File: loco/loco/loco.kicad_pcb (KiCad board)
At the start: 2 copper layers, 26 x 11.4 mm, 4 parts, among them U1 STM32F030F4Px, U2 A4953_LJ, U3 TLV760

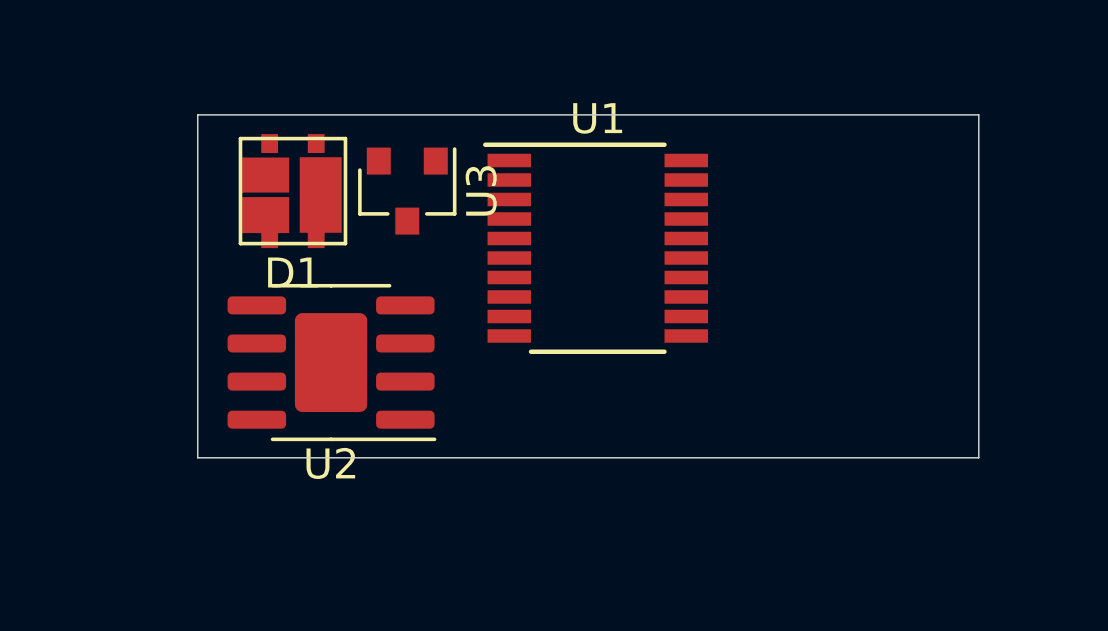
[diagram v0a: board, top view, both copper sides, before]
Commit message: Update
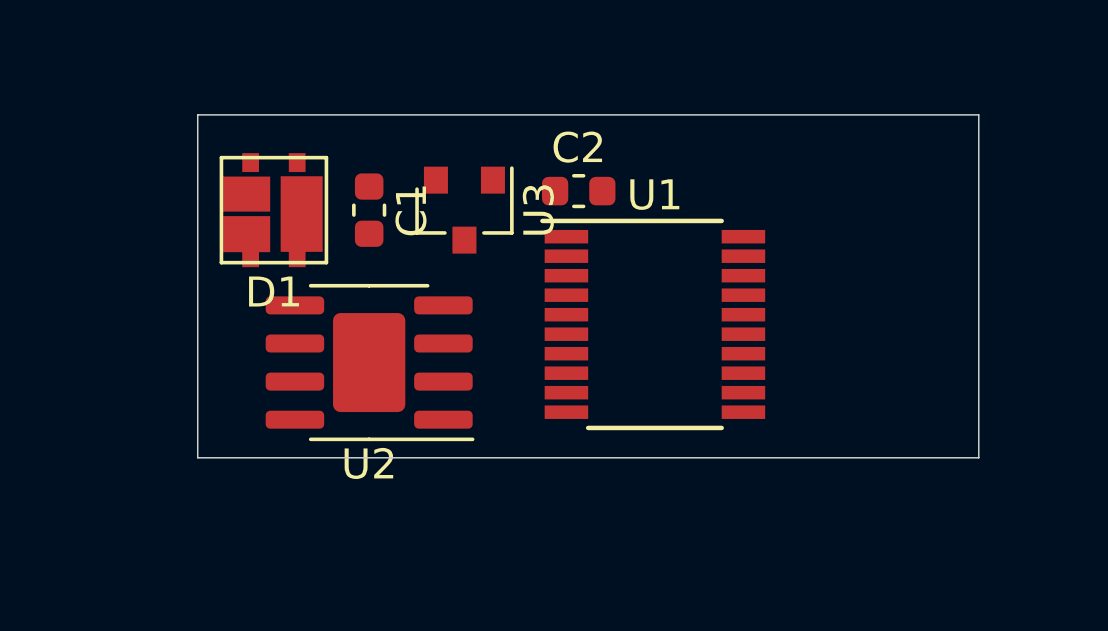
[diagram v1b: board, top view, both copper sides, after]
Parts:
- added C1: C, Capacitor_SMD:C_0603_1608Metric, F.Cu at (121.9, 82.5)
- added C2: C, Capacitor_SMD:C_0603_1608Metric, F.Cu at (128.9, 81.9)
- moved U1 3.18 mm to (131.4, 86.4)
- moved U3 2.01 mm to (125.1, 82.5)
- moved U2 1.27 mm to (121.9, 87.6)
- moved D1 0.90 mm to (118.7, 82.5)
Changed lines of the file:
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@@
     (tracks 0)
     (zones 0)
-    (modules 4)
+    (modules 6)
     (nets 29)
   )
@@
     (add_net RAIL2)
   )
+  (module Capacitor_SMD:C_0603_1608Metric (layer F.Cu)
+    (at 128.905 81.915)
+    (descr "Capacitor SMD 0603 (1608 Metric), square (rectangular) end terminal, IPC_7351 nominal, (Body size source: http://www.tortai-tech.com/upload/download/2011102023233369053.pdf), generated with kicad-footprint-generator")
+    (tags capacitor)
+    (attr smd)
+    (fp_text reference C2 (at 0 -1.43) (layer F.SilkS)
+      (effects (font (size 1 1) (thickness 0.15)))
+    )
+    (fp_text value C (at 0 1.43) (layer F.Fab)
+      (effects (font (size 1 1) (thickness 0.15)))
+    )
+    (fp_text user %R (at 0 0) (layer F.Fab)
+      (effects (font (size 0.4 0.4) (thickness 0.06)))
+    )
+    (fp_line (start 1.48 0.73) (end -1.48 0.73) (layer F.CrtYd) (width 0.05))
+    (fp_line (start 1.48 -0.73) (end 1.48 0.73) (layer F.CrtYd) (width 0.05))
+    (fp_line (start -1.48 -0.73) (end 1.48 -0.73) (layer F.CrtYd) (width 0.05))
+    (fp_line (start -1.48 0.73) (end -1.48 -0.73) (layer F.CrtYd) (width 0.05))
+    (fp_line (start -0.162779 0.51) (end 0.162779 0.51) (layer F.SilkS) (width 0.12))
+    (fp_line (start -0.162779 -0.51) (end 0.162779 -0.51) (layer F.SilkS) (width 0.12))
+    (fp_line (start 0.8 0.4) (end -0.8 0.4) (layer F.Fab) (width 0.1))
+    (fp_line (start 0.8 -0.4) (end 0.8 0.4) (layer F.Fab) (width 0.1))
+    (fp_line (start -0.8 -0.4) (end 0.8 -0.4) (layer F.Fab) (width 0.1))
+    (fp_line (start -0.8 0.4) (end -0.8 -0.4) (layer F.Fab) (width 0.1))
+    (pad 2 smd roundrect (at 0.7875 0) (size 0.875 0.95) (layers F.Cu F.Paste F.Mask) (roundrect_rratio 0.25)
+      (net 16 GND))
+    (pad 1 smd roundrect (at -0.7875 0) (size 0.875 0.95) (layers F.Cu F.Paste F.Mask) (roundrect_rratio 0.25)
+      (net 22 /+3V3))
+    (model ${KISYS3DMOD}/Capacitor_SMD.3dshapes/C_0603_1608Metric.wrl
+      (at (xyz 0 0 0))
+      (scale (xyz 1 1 1))
+      (rotate (xyz 0 0 0))
+    )
+  )
+  (module Capacitor_SMD:C_0603_1608Metric (layer F.Cu)
+    (at 121.92 82.55 270)
+    (descr "Capacitor SMD 0603 (1608 Metric), square (rectangular) end terminal, IPC_7351 nominal, (Body size source: http://www.tortai-tech.com/upload/download/2011102023233369053.pdf), generated with kicad-footprint-generator")
+    (tags capacitor)
+    (attr smd)
+    (fp_text reference C1 (at 0 -1.43 90) (layer F.SilkS)
+      (effects (font (size 1 1) (thickness 0.15)))
+    )
+    (fp_text value C (at 0 1.43 90) (layer F.Fab)
+      (effects (font (size 1 1) (thickness 0.15)))
+    )
+    (fp_text user %R (at 0 0 90) (layer F.Fab)
+      (effects (font (size 0.4 0.4) (thickness 0.06)))
+    )
+    (fp_line (start 1.48 0.73) (end -1.48 0.73) (layer F.CrtYd) (width 0.05))
+    (fp_line (start 1.48 -0.73) (end 1.48 0.73) (layer F.CrtYd) (width 0.05))
+    (fp_line (start -1.48 -0.73) (end 1.48 -0.73) (layer F.CrtYd) (width 0.05))
+    (fp_line (start -1.48 0.73) (end -1.48 -0.73) (layer F.CrtYd) (width 0.05))
+    (fp_line (start -0.162779 0.51) (end 0.162779 0.51) (layer F.SilkS) (width 0.12))
+    (fp_line (start -0.162779 -0.51) (end 0.162779 -0.51) (layer F.SilkS) (width 0.12))
+    (fp_line (start 0.8 0.4) (end -0.8 0.4) (layer F.Fab) (width 0.1))
+    (fp_line (start 0.8 -0.4) (end 0.8 0.4) (layer F.Fab) (width 0.1))
+    (fp_line (start -0.8 -0.4) (end 0.8 -0.4) (layer F.Fab) (width 0.1))
+    (fp_line (start -0.8 0.4) (end -0.8 -0.4) (layer F.Fab) (width 0.1))
+    (pad 2 smd roundrect (at 0.7875 0 270) (size 0.875 0.95) (layers F.Cu F.Paste F.Mask) (roundrect_rratio 0.25)
+      (net 16 GND))
+    (pad 1 smd roundrect (at -0.7875 0 270) (size 0.875 0.95) (layers F.Cu F.Paste F.Mask) (roundrect_rratio 0.25)
+      (net 20 /27V))
+    (model ${KISYS3DMOD}/Capacitor_SMD.3dshapes/C_0603_1608Metric.wrl
+      (at (xyz 0 0 0))
+      (scale (xyz 1 1 1))
+      (rotate (xyz 0 0 0))
+    )
+  )
   (module Package_TO_SOT_SMD:SOT-23 (layer F.Cu)
-    (at 123.19 81.915 270)
+    (at 125.095 82.55 270)
     (descr "SOT-23, Standard")
     (tags SOT-23)
@@
   )
   (module loco:NSR2030 (layer F.Cu)
-    (at 119.38 81.915)
+    (at 118.745 82.55)
     (fp_text reference D1 (at 0 2.75) (layer F.SilkS)
       (effects (font (size 1 1) (thickness 0.15)))
@@
   )
   (module Package_SO:SOIC-8-1EP_3.9x4.9mm_P1.27mm_EP2.41x3.3mm (layer F.Cu)
-    (at 120.65 87.63 180)
+    (at 121.92 87.63 180)
     (descr "SOIC, 8 Pin (http://www.allegromicro.com/~/media/Files/Datasheets/A4950-Datasheet.ashx#page=8), generated with kicad-footprint-generator ipc_gullwing_generator.py")
     (tags "SOIC SO")
@@
   )
   (module Package_SO:TSSOP-20_4.4x6.5mm_P0.65mm (layer F.Cu)
-    (at 129.54 83.82)
+    (at 131.445 86.36)
     (descr "20-Lead Plastic Thin Shrink Small Outline (ST)-4.4 mm Body [TSSOP] (see Microchip Packaging Specification 00000049BS.pdf)")
     (tags "SSOP 0.65")

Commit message: Update
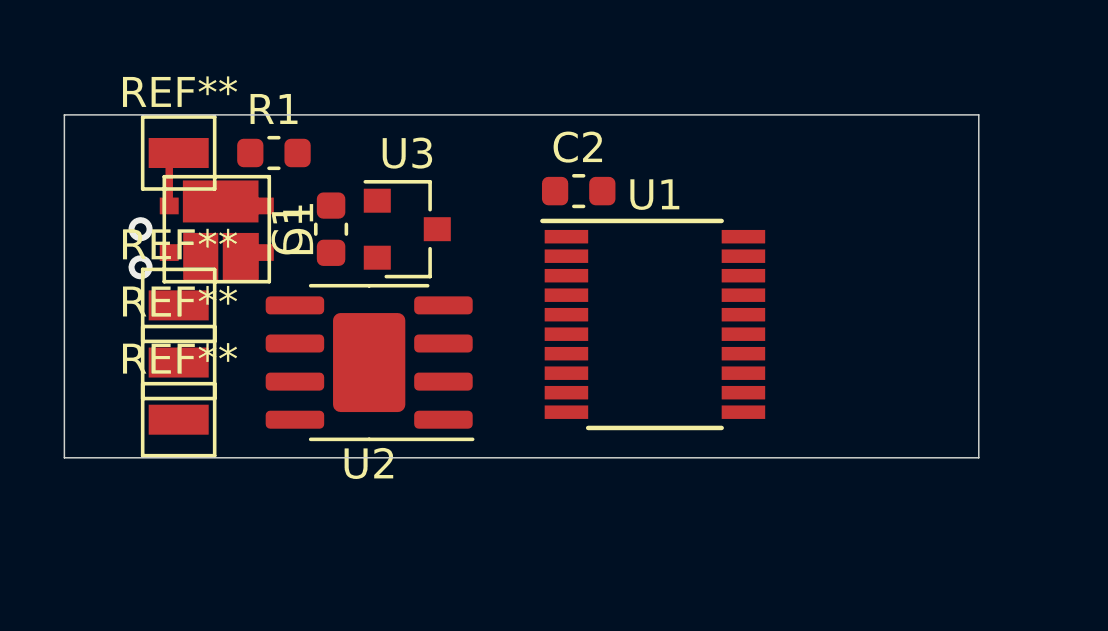
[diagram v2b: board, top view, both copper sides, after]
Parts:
- added R1: TBD, Resistor_SMD:R_0603_1608Metric, F.Cu at (118.7, 80.6)
- added REF**: TestPoint_Pad_2.0x2.0mm, TestPoint:TestPoint_Pad_2.0x2.0mm, F.Cu at (115.6, 80.6)
- added REF**: TestPoint_Pad_2.0x2.0mm, TestPoint:TestPoint_Pad_2.0x2.0mm, F.Cu at (115.6, 85.7)
- added REF**: TestPoint_Pad_2.0x2.0mm, TestPoint:TestPoint_Pad_2.0x2.0mm, F.Cu at (115.6, 87.6)
- added REF**: TestPoint_Pad_2.0x2.0mm, TestPoint:TestPoint_Pad_2.0x2.0mm, F.Cu at (115.6, 89.5)
- moved D1 2.01 mm to (116.8, 83.2), turned to 90 degrees
- moved U3 2.01 mm to (123.2, 83.2), turned to 0 degrees
- moved C1 1.42 mm to (120.7, 83.2), turned to 90 degrees
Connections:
- net Net-(U1-Pad19) renamed /SWDIO
- net Net-(U1-Pad20) renamed /SWCLK
- net Net-(U1-Pad6) renamed /ADC_IN0
- net Net-(U1-Pad7) renamed /ADC_IN1
- net Net-(U1-Pad8) renamed /ADC_IN3
- net Net-(U1-Pad9) renamed /ADC_IN4
- U1 pad 10: Net-(U1-Pad10) -> /TIM14_CH1
- U1 pad 12: Net-(U1-Pad12) -> /TIM3_CH1
- U1 pad 13: Net-(U1-Pad13) -> /TIM3_CH2
- U2 pad 2: /IN2 -> /TIM3_CH1
- U2 pad 3: /IN1 -> /TIM3_CH2
- U2 pad 6: /M1 -> M1
- U2 pad 8: /M2 -> M2
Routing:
- net RAIL2: track 0.00 -> 1.90 mm
- net /27V: track 0.00 -> 1.52 mm
- net GND: vias 0 -> 2
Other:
- board size 26 x 11.4 mm -> 30.5 x 11.4 mm

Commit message: FR and RL
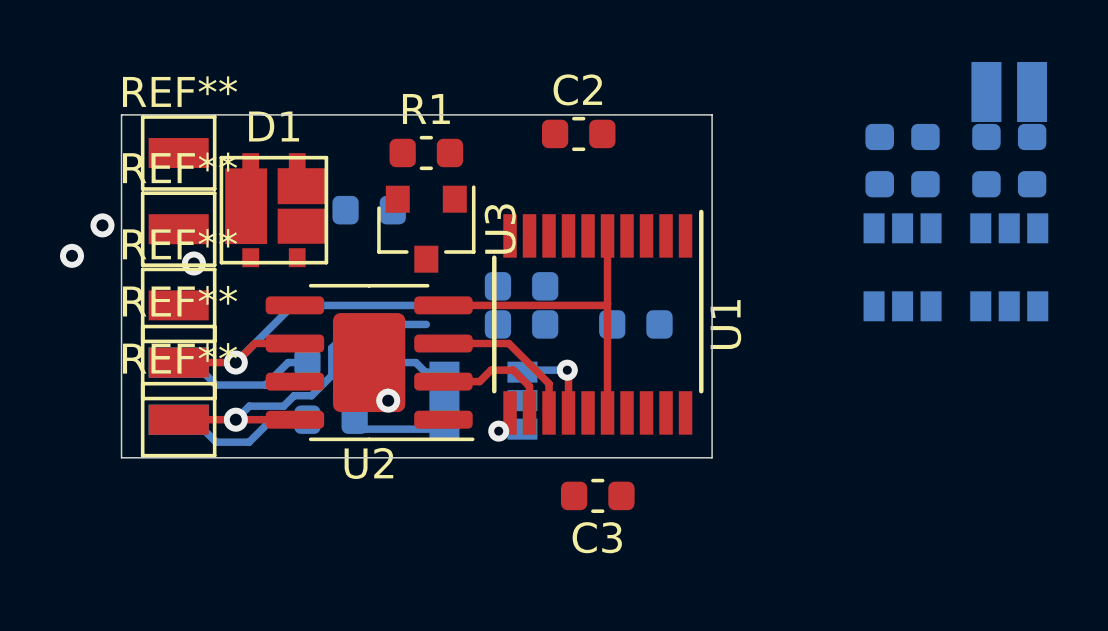
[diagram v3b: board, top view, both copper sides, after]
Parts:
- added C3: C, Capacitor_SMD:C_0603_1608Metric, F.Cu at (129.5, 92.1)
- added C4: 100n, Capacitor_SMD:C_0603_1608Metric, B.Cu at (130.8, 86.4)
- added Q1: FDC6561AN, Package_TO_SOT_SMD:SuperSOT-6, B.Cu at (143.3, 84.5)
- added Q2: FDC6561AN, Package_TO_SOT_SMD:SuperSOT-6, B.Cu at (139.7, 84.5)
- added Q3: FDC6561AN, Package_TO_SOT_SMD:SuperSOT-6, B.Cu at (125.7, 88.9)
- added R2: 10K, Resistor_SMD:R_0603_1608Metric, B.Cu at (127.0, 85.1)
- added R3: 10K, Resistor_SMD:R_0603_1608Metric, B.Cu at (127.0, 86.4)
- added R4: TBD, Resistor_SMD:R_0603_1608Metric, B.Cu at (144.0, 80.9)
- added R5: TBD, Resistor_SMD:R_0603_1608Metric, B.Cu at (142.5, 80.9)
- added R6: TBD, Resistor_SMD:R_0603_1608Metric, B.Cu at (140.5, 80.9)
- added R7: TBD, Resistor_SMD:R_0603_1608Metric, B.Cu at (138.9, 80.9)
- added R8: TBD, Resistor_SMD:R_0603_1608Metric, B.Cu at (120.7, 87.6)
- added R9: TBD, Resistor_SMD:R_0603_1608Metric, B.Cu at (120.7, 89.5)
- added REF**: TestPoint_Pad_2.0x2.0mm, TestPoint:TestPoint_Pad_2.0x2.0mm, B.Cu at (115.6, 89.5)
- added REF**: TestPoint_Pad_2.0x2.0mm, TestPoint:TestPoint_Pad_2.0x2.0mm, B.Cu at (115.6, 87.6)
- added REF**: TestPoint_Pad_2.0x2.0mm, TestPoint:TestPoint_Pad_2.0x2.0mm, F.Cu at (115.6, 83.2)
- added REF**: TestPoint_Pad_2.0x2.0mm, TestPoint:TestPoint_Pad_2.0x2.0mm, B.Cu at (142.5, 78.6)
- added REF**: TestPoint_Pad_2.0x2.0mm, TestPoint:TestPoint_Pad_2.0x2.0mm, B.Cu at (144.0, 78.6)
- C1: moved to B.Cu
- moved R1 5.08 mm to (123.8, 80.6)
- moved REF** 5.08 mm to (115.6, 85.7)
- moved REF** 5.08 mm to (115.6, 80.6)
- moved D1 2.01 mm to (118.7, 82.5), turned to 180 degrees
- moved C2 1.91 mm to (128.9, 80.0)
- moved U1 1.91 mm to (129.5, 86.4), turned to 270 degrees
- moved C1 1.42 mm to (121.9, 82.5), turned to 0 degrees
- moved U3 0.64 mm to (123.8, 83.2), turned to 270 degrees
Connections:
- R1 pad 1: RAIL2 -> RAIL1
- U1 pad 11: Net-(U1-Pad11) -> /_RL
- U1 pad 14: Net-(U1-Pad14) -> /_FL
- U2 pad 4: Net-(U2-Pad4) -> /+3V3
- U2 pad 7: Net-(U2-Pad7) -> GND
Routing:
- net M2: track 0.00 -> 12.1 mm, vias 0 -> 1
- net /+3V3: track 0.00 -> 11.4 mm
- net M1: track 0.00 -> 11.3 mm, vias 0 -> 1
- net /TIM3_CH2: track 0.00 -> 5.05 mm
- net RL: track 0.00 -> 4.91 mm
- net FL: track 0.00 -> 4.91 mm
- net /TIM3_CH1: track 0.00 -> 4.14 mm
- net Net-(Q3-Pad4): track 0.00 -> 3.15 mm
- net Net-(Q3-Pad6): track 0.00 -> 3.13 mm
- net /_FL: track 0.00 -> 2.96 mm, vias 0 -> 1
- net RAIL2: track 1.90 -> 0.00 mm
- net /_RL: track 0.00 -> 1.58 mm, vias 0 -> 1
- net /27V: track 1.52 -> 0.00 mm, vias 0 -> 1
- net GND: vias 2 -> 3
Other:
- board size 30.5 x 11.4 mm -> 19.7 x 11.4 mm

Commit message: F1 and F2
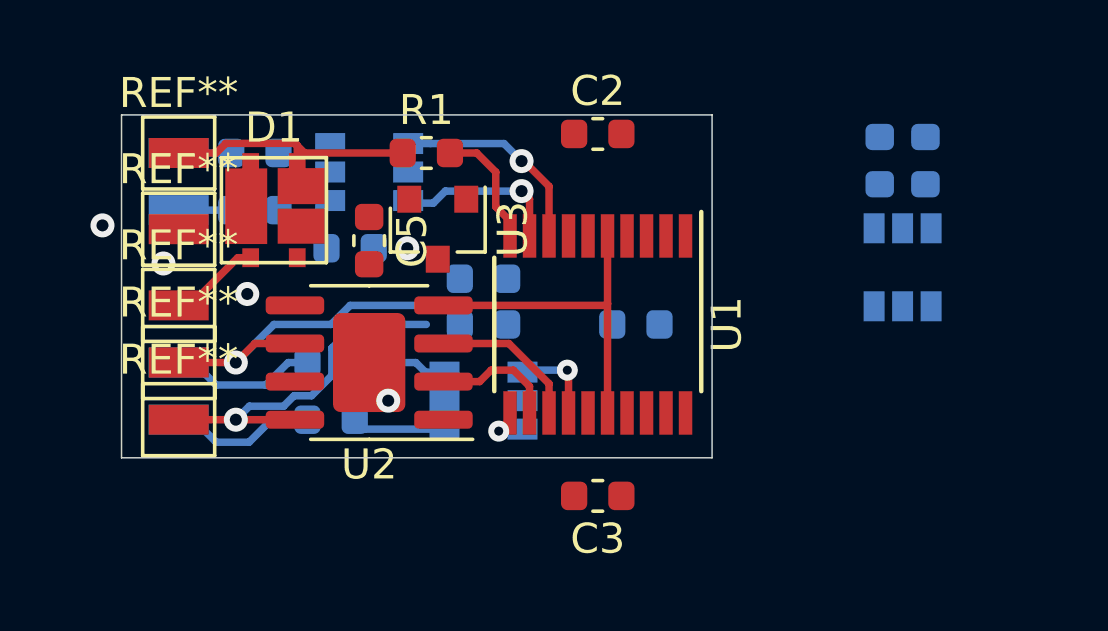
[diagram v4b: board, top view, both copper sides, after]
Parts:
- added C5: C, Capacitor_SMD:C_0603_1608Metric, F.Cu at (121.9, 83.6)
- moved REF** 28.5 mm to (115.6, 80.6), turned to 180 degrees
- moved REF** 27.2 mm to (115.6, 82.5), turned to 180 degrees
- moved R4 25.9 mm to (118.1, 80.6), turned to 180 degrees
- moved R5 24.4 mm to (118.1, 82.5), turned to 180 degrees
- moved Q1 21.6 mm to (121.9, 81.3), turned to 180 degrees
- moved C1 1.42 mm to (121.3, 83.8)
- moved R2 1.30 mm to (125.7, 84.8)
- moved R3 1.27 mm to (125.7, 86.4)
- moved C2 0.63 mm to (129.5, 80.0)
- moved U3 0.38 mm to (124.2, 83.2)
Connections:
- Q1 pad 1: Net-(Q1-Pad1) -> /_F1
- Q1 pad 3: Net-(Q1-Pad3) -> /_F2
- U1 pad 8: /ADC_IN3 -> /_F1
- U1 pad 9: /ADC_IN4 -> /_F2
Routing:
- net RAIL1: track 0.00 -> 8.30 mm
- net /_F1: track 0.00 -> 6.94 mm, vias 0 -> 1
- net /_F2: track 0.00 -> 5.59 mm, vias 0 -> 1
- net /TIM14_CH1: track 0.00 -> 4.12 mm
- net RAIL2: track 0.00 -> 3.06 mm
- net F2: track 0.00 -> 1.75 mm
- net F1: track 0.00 -> 1.75 mm
- net /27V: vias 1 -> 2

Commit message: Docs added
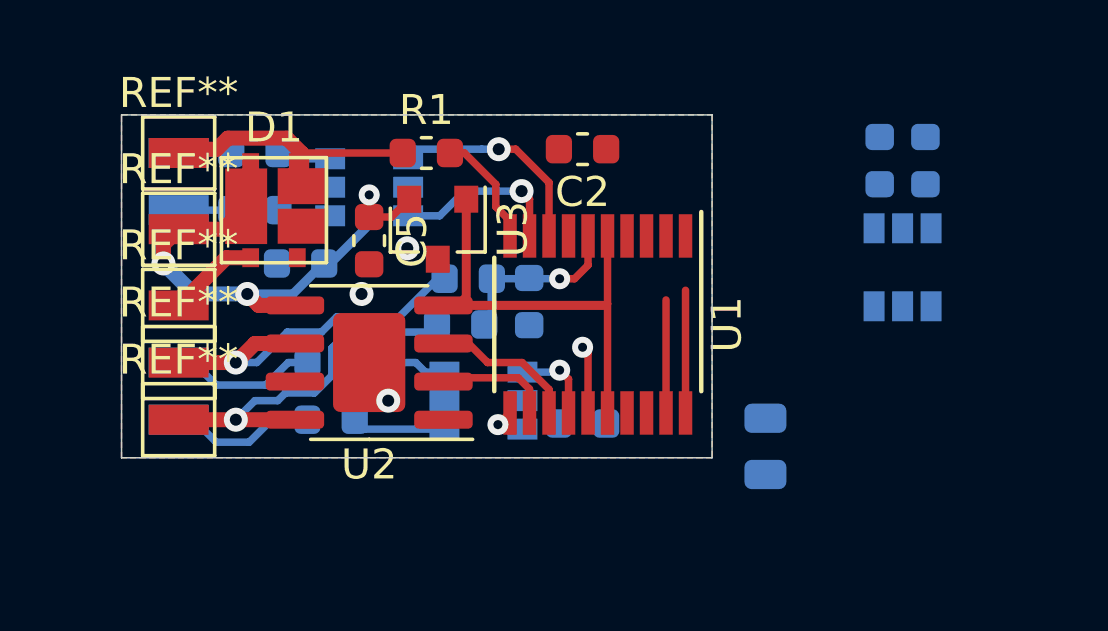
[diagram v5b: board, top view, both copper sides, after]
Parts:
- added C6: 2u2, Capacitor_SMD:C_0805_2012Metric, B.Cu at (135.1, 90.4)
- C3: moved to B.Cu
- moved C4 3.64 mm to (127.3, 85.6), turned to 270 degrees
- moved C3 2.47 mm to (129.0, 89.7)
- moved C1 1.73 mm to (119.6, 84.3), turned to 180 degrees
- moved R3 0.76 mm to (125.0, 86.4)
- moved C2 0.72 mm to (129.0, 80.5), turned to 180 degrees
- moved R2 0.51 mm to (125.2, 84.8)
- moved Q1 0.51 mm to (121.9, 81.8)
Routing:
- net /27V: track 0.00 -> 18.5 mm, vias 2 -> 3
- net /ADC_IN0: track 0.00 -> 6.03 mm, vias 0 -> 1
- net /+3V3: track 11.4 -> 15.5 mm
- net /SWCLK: track 0.00 -> 4.09 mm
- net /SWDIO: track 0.00 -> 3.77 mm
- net GND: track 0.00 -> 2.26 mm, vias 3 -> 4
- net Net-(Q1-Pad6): track 0.00 -> 1.80 mm
- net Net-(Q1-Pad4): track 0.00 -> 1.80 mm
- net RAIL1: track 8.30 -> 9.73 mm
- net M1: track 11.3 -> 12.3 mm
- added copper zone on B.Cu, net GND
- added copper zone on F.Cu, net GND

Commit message: Routing done, mostly
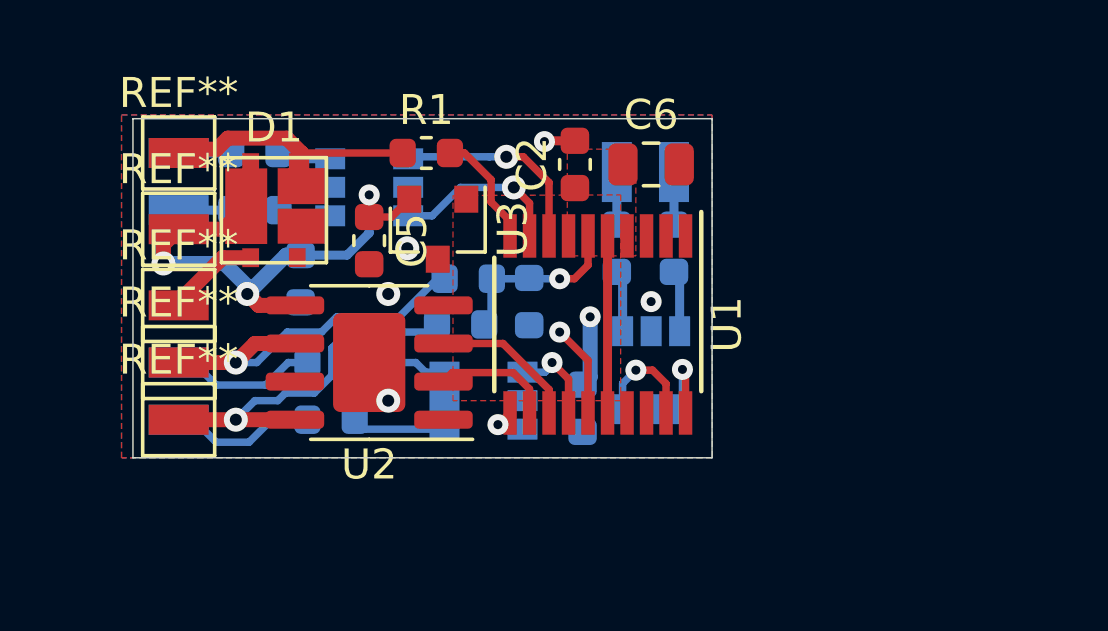
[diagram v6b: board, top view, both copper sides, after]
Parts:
- added REF**: TestPoint_Pad_2.0x2.0mm, TestPoint:TestPoint_Pad_2.0x2.0mm, B.Cu at (130.2, 81.3)
- added REF**: TestPoint_Pad_2.0x2.0mm, TestPoint:TestPoint_Pad_2.0x2.0mm, B.Cu at (132.1, 81.3)
- C6: moved to F.Cu
- moved C6 10.1 mm to (131.3, 81.0), turned to 0 degrees
- moved R7 9.24 mm to (130.2, 83.8)
- moved Q2 9.06 mm to (131.3, 87.9)
- moved R6 8.88 mm to (132.1, 83.8)
- moved C2 0.57 mm to (128.8, 81.0), turned to 90 degrees
- moved C3 0.51 mm to (129.0, 89.2), turned to 270 degrees
- moved C1 0.51 mm to (119.6, 84.8), turned to 270 degrees
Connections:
- Q2 pad 1: Net-(Q2-Pad1) -> /SWCLK
- Q2 pad 3: Net-(Q2-Pad3) -> /SWDIO
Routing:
- net /+3V3: track 15.5 -> 8.71 mm, vias 0 -> 1
- net Net-(Q2-Pad4): track 0.00 -> 2.06 mm
- net Net-(Q2-Pad6): track 0.00 -> 2.05 mm
- net GND: track 2.26 -> 4.11 mm, vias 4 -> 6
- net F4: track 0.00 -> 1.75 mm
- net F3: track 0.00 -> 1.75 mm
- net /SWCLK: track 4.09 -> 2.86 mm, vias 0 -> 1
- net /27V: track 18.5 -> 19.0 mm
- net /SWDIO: track 3.77 -> 3.65 mm, vias 0 -> 1
- added copper zone on F.Cu, net /+3V3
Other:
- board size 19.7 x 11.4 mm -> 19.3 x 11.3 mm
